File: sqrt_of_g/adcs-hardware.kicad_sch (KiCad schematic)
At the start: 18 parts, among them J10 35362-0650, J11 Conn_01x20, J13 35362-0650, J15 353620850, J16 35362-0650, J18 35362-0650, J19 353621050, J20 353621050, J7 Conn_01x08, J8 Conn_01x20, J9 35362-0650, Q1 IRLML2803, Q2 NDS8434

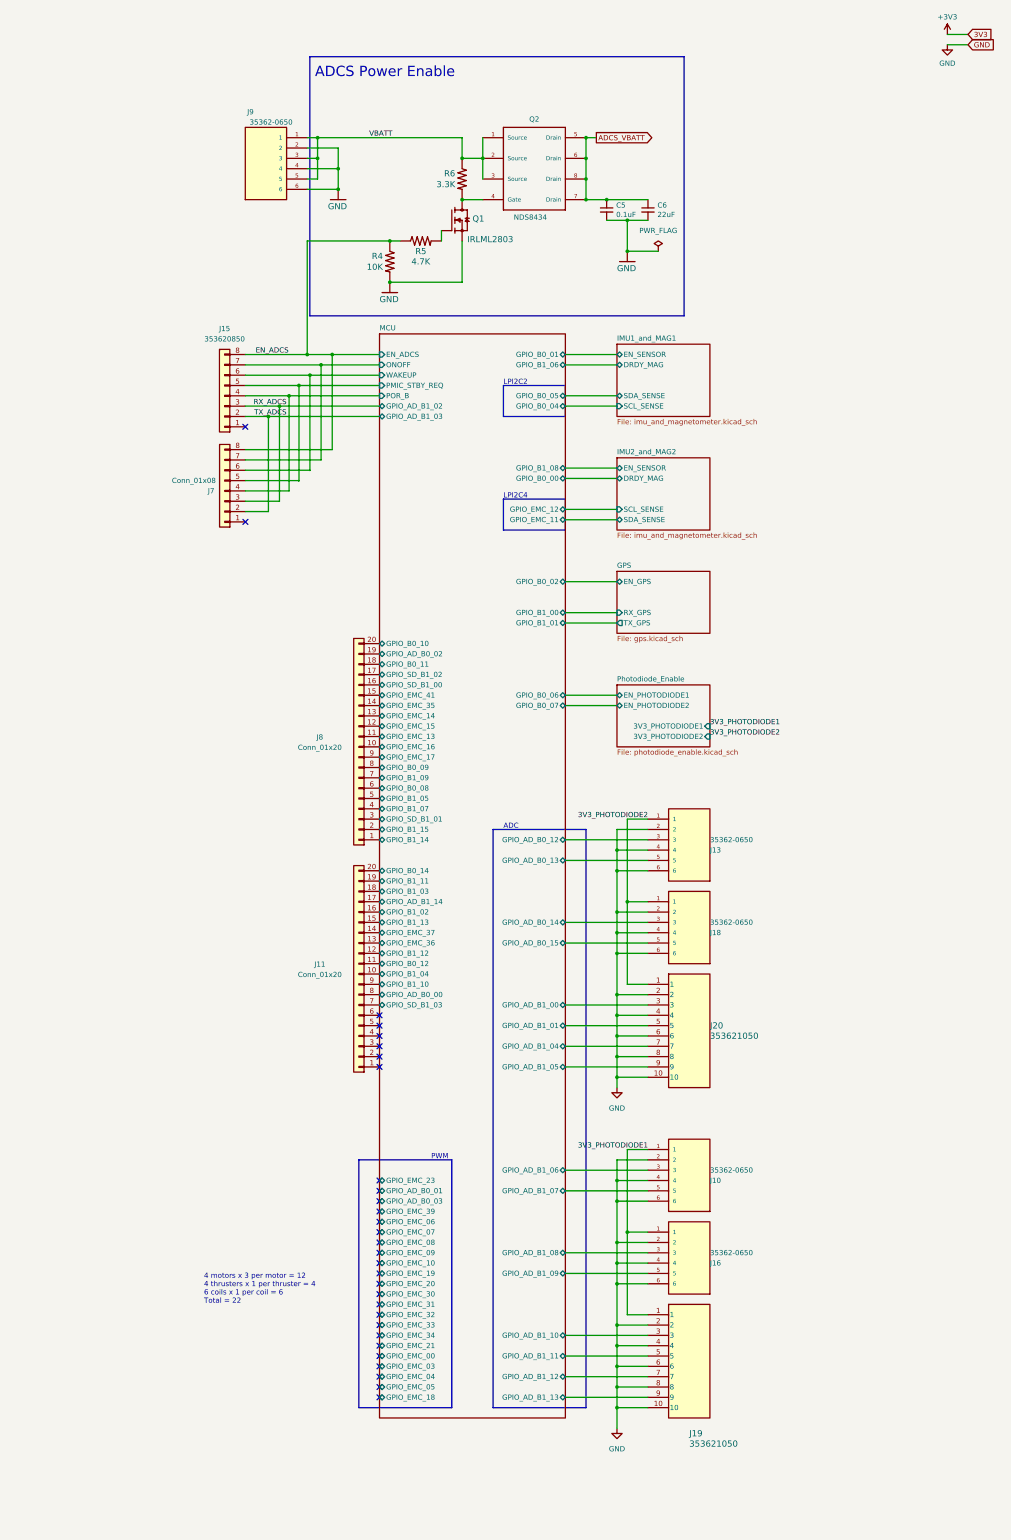
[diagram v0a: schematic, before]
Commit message: ready for 2nd round of reviews
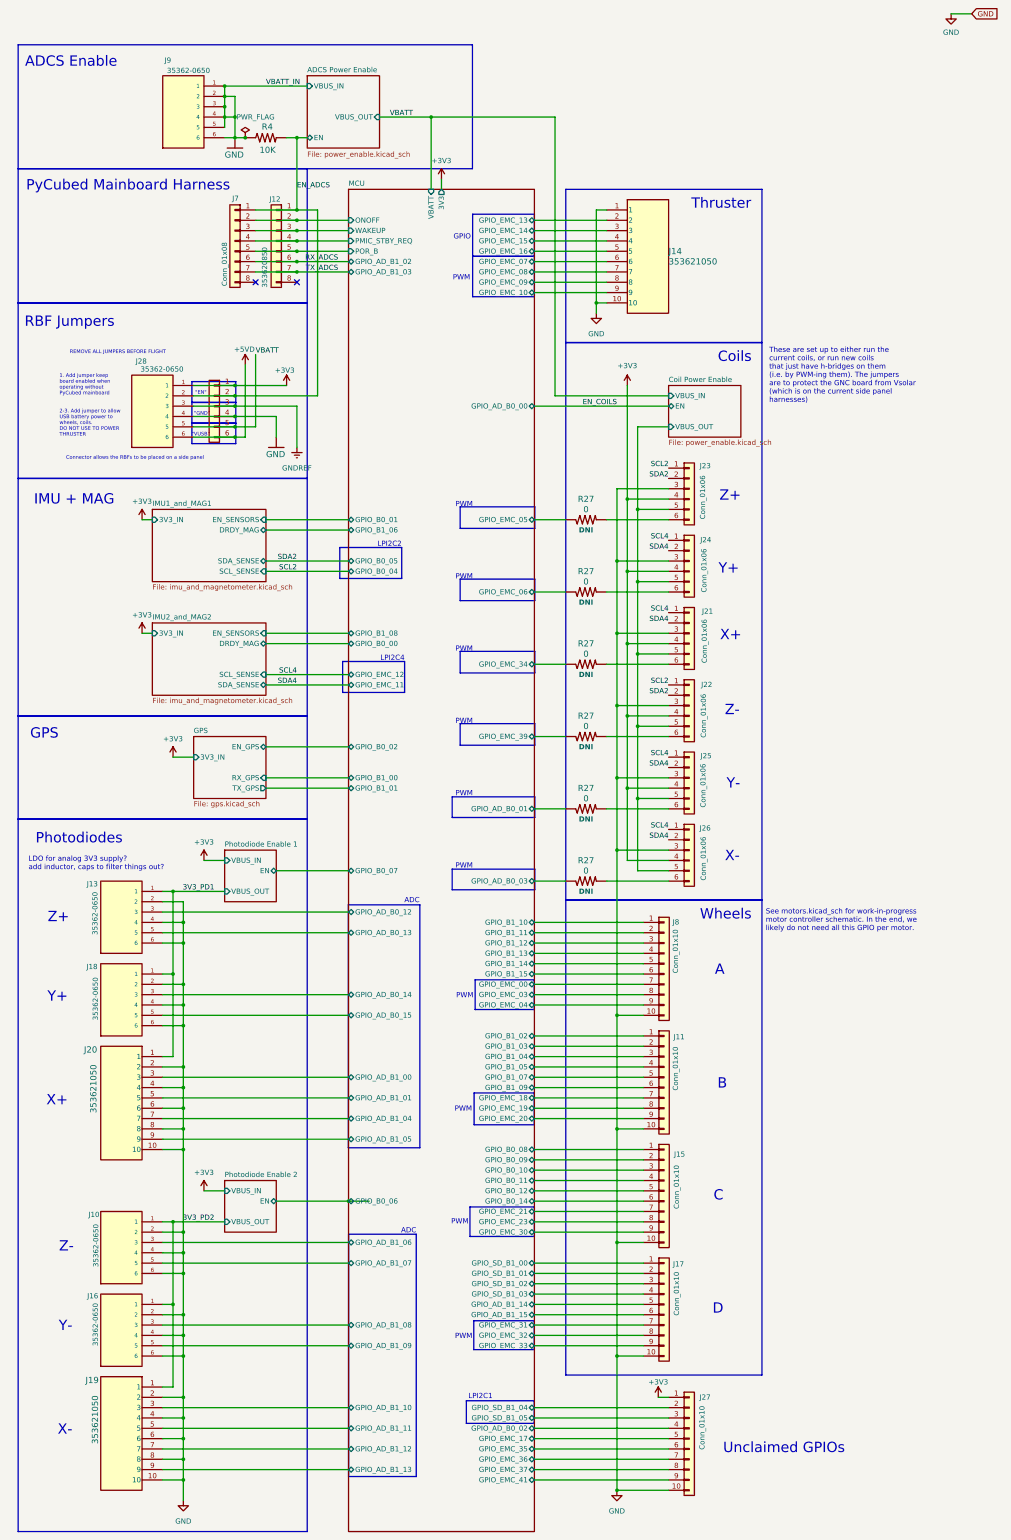
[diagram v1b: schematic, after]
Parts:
- removed C5: 0.1uF, Capacitor_SMD:C_0603_1608Metric, symbol Device:C_Small
- removed C6: 22uF, Capacitor_SMD:C_0603_1608Metric, symbol Device:C_Small
- removed J11, J8: Conn_01x20, symbol Connector_Generic:Conn_01x20
- removed J15: 353620850, mainboard:353620850, symbol Connector_Generic:Conn_01x08
- removed Q1: IRLML2803, mainboard:SOT-23, symbol mainboard:IRLML2803TRPBF
- removed Q2: NDS8434, mainboard:NDS8434, symbol mainboard:NDS8434
- removed R5: 4.7K, Resistor_SMD:R_0603_1608Metric, symbol mainboard:R-US_R0603
- removed R6: 3.3K, Resistor_SMD:R_0603_1608Metric, symbol mainboard:R-US_R0603
- added J11, J15, J17, J27, J8: Conn_01x10, symbol Connector_Generic:Conn_01x10
- added J12: 353620850, mainboard:353620850, symbol Connector_Generic:Conn_01x08
- added J14: 353621050, CON_353621050, symbol adcs:353621050
- added J21, J22, J23, J24, J25, J26: Conn_01x06, symbol Connector_Generic:Conn_01x06
- added J28: 35362-0650, mainboard:MOLEX_35362-0650, symbol mainboard:35362-0650
- added J6: Conn_01x06, Connector_PinHeader_2.54mm:PinHeader_1x06_P2.54mm_Vertical, symbol Connector_Generic:Conn_01x06
- added R27 (x6): 0, Resistor_SMD:R_0603_1608Metric, symbol mainboard:R-US_R0603
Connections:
- net +3V3: now also J21.4 (Pin_4), J22.4 (Pin_4), J23.4 (Pin_4), J24.4 (Pin_4), J25.4 (Pin_4), J26.4 (Pin_4), J27.1 (Pin_1), J28.1, J6.1 (Pin_1)
- net EN_ADCS: now also J7.1 (Pin_1), R4.2, J12.1 (Pin_1), J28.2, J6.2 (Pin_2); no longer J7.8 (Pin_8), R4.1
- net GND: now also J9.1, J9.3, J9.5, R4.1, J11.10 (Pin_10), J14.1, J14.10, J15.10 (Pin_10), J17.10 (Pin_10), J21.3 (Pin_3), J22.3 (Pin_3), J23.3 (Pin_3), J24.3 (Pin_3), J25.3 (Pin_3), J26.3 (Pin_3), J27.10 (Pin_10), J28.4, J6.4 (Pin_4), J8.10 (Pin_10); no longer R4.2
- net MCU/GPIO_AD_B0_01: now also R27.1
- net MCU/GPIO_AD_B0_02: now also J27.4 (Pin_4)
- net MCU/GPIO_AD_B0_03: now also R27.1
- net MCU/GPIO_AD_B1_14: now also J17.5 (Pin_5)
- net MCU/GPIO_B0_08: now also J15.1 (Pin_1)
- net MCU/GPIO_B0_09: now also J15.2 (Pin_2)
- net MCU/GPIO_B0_10: now also J15.3 (Pin_3)
- net MCU/GPIO_B0_11: now also J15.4 (Pin_4)
- net MCU/GPIO_B0_12: now also J15.5 (Pin_5)
- net MCU/GPIO_B0_14: now also J15.6 (Pin_6)
- net MCU/GPIO_B1_02: now also J11.1 (Pin_1)
- net MCU/GPIO_B1_03: now also J11.2 (Pin_2)
- net MCU/GPIO_B1_04: now also J11.3 (Pin_3)
- net MCU/GPIO_B1_05: now also J11.4 (Pin_4)
- net MCU/GPIO_B1_07: now also J11.5 (Pin_5)
- net MCU/GPIO_B1_09: now also J11.6 (Pin_6)
- net MCU/GPIO_B1_10: now also J8.1 (Pin_1)
- net MCU/GPIO_B1_11: now also J8.2 (Pin_2)
- net MCU/GPIO_B1_12: now also J8.3 (Pin_3)
- net MCU/GPIO_B1_13: now also J8.4 (Pin_4)
- net MCU/GPIO_B1_14: now also J8.5 (Pin_5)
- net MCU/GPIO_B1_15: now also J8.6 (Pin_6)
- net MCU/GPIO_EMC_00: now also J8.7 (Pin_7)
- net MCU/GPIO_EMC_03: now also J8.8 (Pin_8)
- net MCU/GPIO_EMC_04: now also J8.9 (Pin_9)
- net MCU/GPIO_EMC_05: now also R27.1
- net MCU/GPIO_EMC_06: now also R27.1
- net MCU/GPIO_EMC_07: now also J14.6
- net MCU/GPIO_EMC_08: now also J14.7
- net MCU/GPIO_EMC_09: now also J14.8
- net MCU/GPIO_EMC_10: now also J14.9
- net MCU/GPIO_EMC_13: now also J14.2
- net MCU/GPIO_EMC_14: now also J14.3
- net MCU/GPIO_EMC_15: now also J14.4
- net MCU/GPIO_EMC_16: now also J14.5
- net MCU/GPIO_EMC_17: now also J27.5 (Pin_5)
- net MCU/GPIO_EMC_18: now also J11.7 (Pin_7)
- net MCU/GPIO_EMC_19: now also J11.8 (Pin_8)
- net MCU/GPIO_EMC_20: now also J11.9 (Pin_9)
- net MCU/GPIO_EMC_21: now also J15.7 (Pin_7)
- net MCU/GPIO_EMC_23: now also J15.8 (Pin_8)
- net MCU/GPIO_EMC_30: now also J15.9 (Pin_9)
- net MCU/GPIO_EMC_31: now also J17.7 (Pin_7)
- net MCU/GPIO_EMC_32: now also J17.8 (Pin_8)
- net MCU/GPIO_EMC_33: now also J17.9 (Pin_9)
- net MCU/GPIO_EMC_34: now also R27.1
- net MCU/GPIO_EMC_35: now also J27.6 (Pin_6)
- net MCU/GPIO_EMC_36: now also J27.7 (Pin_7)
- net MCU/GPIO_EMC_37: now also J27.8 (Pin_8)
- net MCU/GPIO_EMC_39: now also R27.1
- net MCU/GPIO_EMC_41: now also J27.9 (Pin_9)
- net MCU/GPIO_SD_B1_00: now also J17.1 (Pin_1)
- net MCU/GPIO_SD_B1_01: now also J17.2 (Pin_2)
- net MCU/GPIO_SD_B1_02: now also J17.3 (Pin_3)
- net MCU/GPIO_SD_B1_03: now also J17.4 (Pin_4)
- net MCU/ONOFF: now also J7.2 (Pin_2), J12.2 (Pin_2); no longer J7.7 (Pin_7)
- net MCU/PMIC_STBY_REQ: now also J7.4 (Pin_4), J12.4 (Pin_4); no longer J7.5 (Pin_5)
- net MCU/POR_B: now also J7.5 (Pin_5), J12.5 (Pin_5); no longer J7.4 (Pin_4)
- net MCU/WAKEUP: now also J7.3 (Pin_3), J12.3 (Pin_3); no longer J7.6 (Pin_6)
- net RX_ADCS: now also J7.6 (Pin_6), J12.6 (Pin_6); no longer J7.3 (Pin_3)
- net TX_ADCS: now also J7.7 (Pin_7), J12.7 (Pin_7); no longer J7.2 (Pin_2)
- net VBATT: now also J28.5, J6.5 (Pin_5); no longer J9.1, J9.3, J9.5
- net 3V3_PHOTODIODE1 renamed 3V3_PD2
- net 3V3_PHOTODIODE2 renamed 3V3_PD1
- new net: J25.6 (Pin_6), R27.2
- new net: J26.6 (Pin_6), R27.2
- new net: J24.6 (Pin_6), R27.2
- new net: J23.6 (Pin_6), R27.2
- new net: J21.6 (Pin_6), R27.2
- new net: J22.6 (Pin_6), R27.2
- new net +5VD: J28.6, J6.6 (Pin_6)
- new net Coil Power Enable/VBUS_OUT: J21.5 (Pin_5), J22.5 (Pin_5), J23.5 (Pin_5), J24.5 (Pin_5), J25.5 (Pin_5), J26.5 (Pin_5)
- new net GNDREF: J28.3, J6.3 (Pin_3)
- new net MCU/GPIO_AD_B1_15: J17.6 (Pin_6)
- new net MCU/GPIO_SD_B1_04: J27.2 (Pin_2)
- new net MCU/GPIO_SD_B1_05: J27.3 (Pin_3)
- new net SCL2: J22.1 (Pin_1), J23.1 (Pin_1)
- new net SCL4: J21.1 (Pin_1), J24.1 (Pin_1), J25.1 (Pin_1), J26.1 (Pin_1)
- new net SDA2: J22.2 (Pin_2), J23.2 (Pin_2)
- new net SDA4: J21.2 (Pin_2), J24.2 (Pin_2), J25.2 (Pin_2), J26.2 (Pin_2)
- no-connect marks 30 -> 2
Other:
- removed sheet Photodiode_Enable
- added sheet ADCS Power Enable (power_enable.kicad_sch)
- added sheet Coil Power Enable (power_enable.kicad_sch)
- added sheet Photodiode Enable 1 (power_enable.kicad_sch)
- added sheet Photodiode Enable 2 (power_enable.kicad_sch)
- sheet GPS ports: added 3V3_IN; removed none
- sheet IMU1_and_MAG1 ports: added 3V3_IN, EN_SENSORS; removed EN_SENSOR
- sheet IMU2_and_MAG2 ports: added 3V3_IN, EN_SENSORS; removed EN_SENSOR
- sheet MCU ports: added 3V3, GPIO_AD_B1_15, GPIO_SD_B1_04, GPIO_SD_B1_05, VBATT; removed EN_ADCS
- note added: ""EN""
- note added: ""GND""
- note added: ""VUSB""
- note added: "1. Add jumper keep board enabled when operating without PyCubed mainboard"
- note added: "2-3. Add jumper to allow USB battery power to wheels, coils. DO NOT USE TO POWER THRUSTER"
- note added: "A"
- note added: "ADCS Enable"
- note added: "B"
- note added: "C"
- note added: "Coils"
- note added: "Connector allows the RBFs to be placed on a side panel"
- note added: "D"
- note added: "GPIO"
- note added: "GPS"
- note added: "IMU + MAG"
- note added: "LDO for analog 3V3 supply? add inductor, caps to filter things out?"
- note added: "LPI2C1"
- note added: "Photodiodes"
- note added: "PyCubed Mainboard Harness"
- note added: "RBF Jumpers"
- note added: "REMOVE ALL JUMPERS BEFORE FLIGHT"
- note added: "See motors.kicad_sch for work-in-progress motor controller schematic. In the end, we likely do not need all this GPIO per motor."
- note added: "These are set up to either run the current coils, or run new coils that just have h-bridges on them (i.e. by PWM-ing them). The jumpers are to protect the GNC board from Vsolar (which is on the current side panel harnesses)"
- note added: "Thruster"
- note added: "Unclaimed GPIOs"
- note added: "Wheels"
- note added: "X+"
- note added: "X-"
- note added: "Y+"
- note added: "Y-"
- note added: "Z+"
- note added: "Z-"
- note removed: "4 motors x 3 per motor = 12 4 thrusters x 1 per thruster = 4 6 coils x 1 per coil = 6 Total = 22"
- note removed: "ADCS Power Enable"
- moved on the sheet: J10, J13, J16, J18, J19, J20, J9, R4
